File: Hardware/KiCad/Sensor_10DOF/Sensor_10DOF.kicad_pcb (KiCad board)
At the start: 2 copper layers, 29.2 x 37 mm, 21 parts, among them U1 BMI160, U2 BME280, U3 LSM303AGR, U4 WeMos_D1_mini, U6 LP2985-3.3

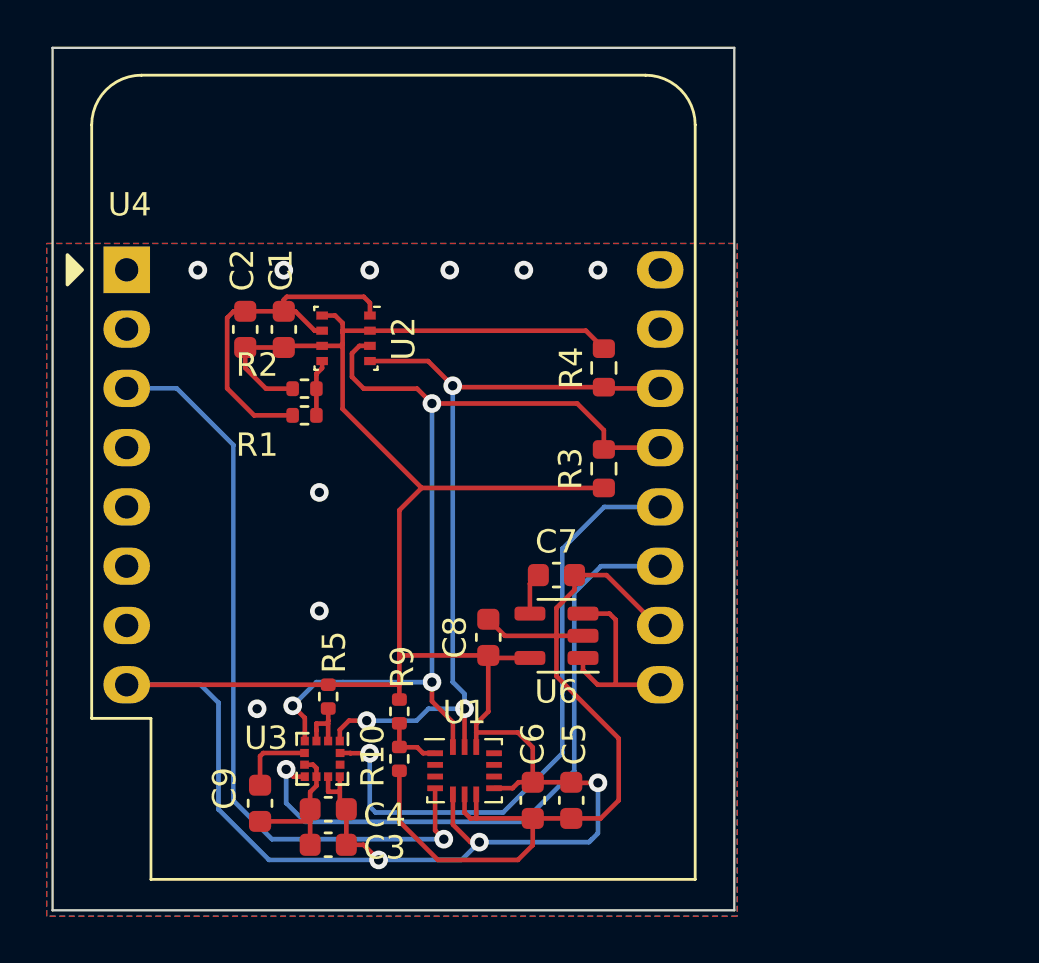
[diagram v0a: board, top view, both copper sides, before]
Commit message: fast fertig. Pinbelegung prüfen
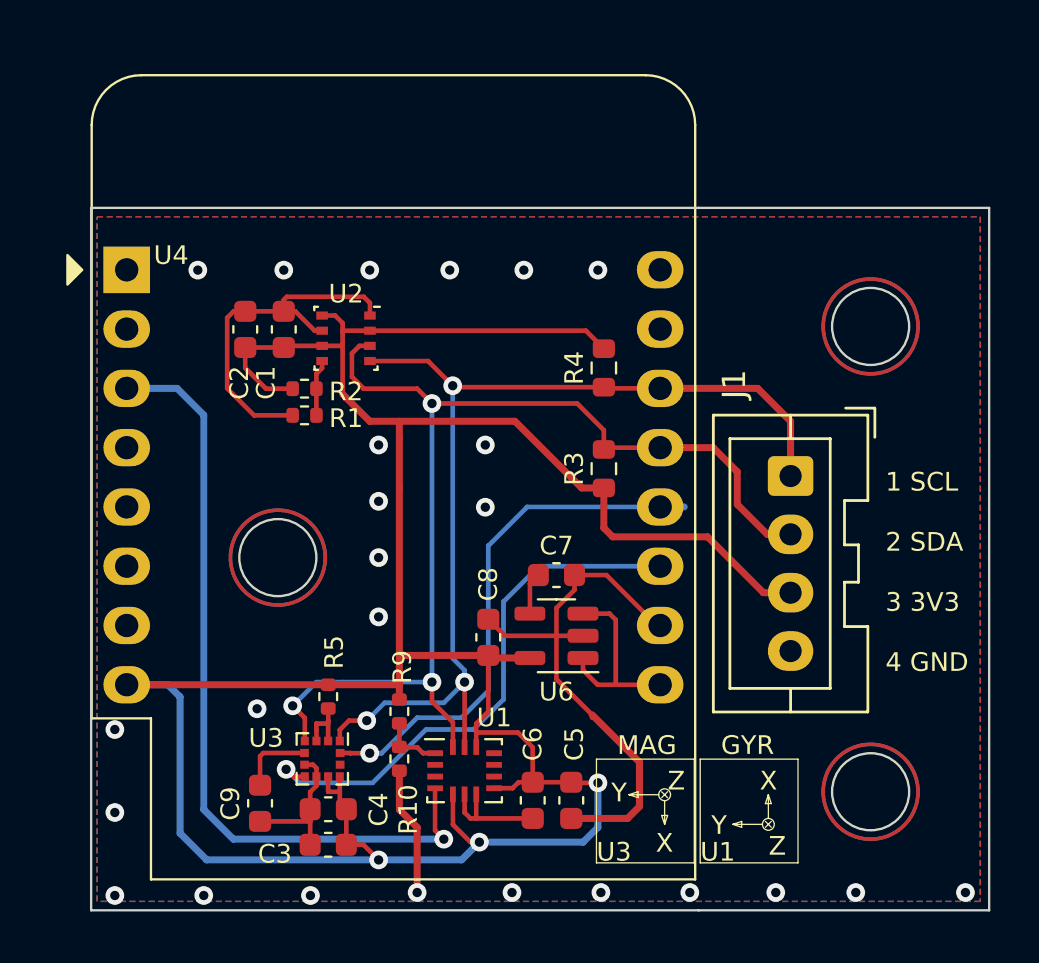
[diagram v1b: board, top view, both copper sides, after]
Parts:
- added J1: Conn_01x04, Connector_JST:JST_XA_B04B-XASK-1_1x04_P2.50mm_Vertical, F.Cu at (132.0, 93.3)
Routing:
- net +3.3V: track 113.5 -> 127.0 mm
- net /SCL: track 34.8 -> 44.6 mm
- net /SDA: track 40.1 -> 48.6 mm
- net GND: track 60.7 -> 56.1 mm, vias 9 -> 25
- net /INT_M: track 27.7 -> 23.5 mm
- net /INT_XL: track 26.7 -> 22.8 mm
- net /INT_A: track 32.9 -> 33.8 mm
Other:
- board size 29.2 x 37 mm -> 38.5 x 30.1 mm
- board text added: "1 SCL 2 SDA 3 3V3 4 GND"
- board text added: "GYR"
- board text added: "MAG"
- board text added: "SENSOR 10DOF BMI160/323 LSM303AGR BME280"
- board text added: "U1"
- board text added: "U3"
- board text added: "X"
- board text added: "Y"
- board text added: "Z"
